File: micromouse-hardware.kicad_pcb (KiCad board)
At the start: 2 copper layers, 51 parts, among them Q1 MBT3904DW1, Q2 MBT3904DW1, Q3 MBT3904DW1, Q4 TEFT4300, Q5 TEFT4300, Q6 TEFT4300, Q7 TEFT4300, Q8 TEFT4300, SW1 SLW-116641-5A-S-D, SW2 SW_DIP_x02, U1 DRV8833PWPR, U2 74HC4051, U3 74HC238D, U4 MT3608

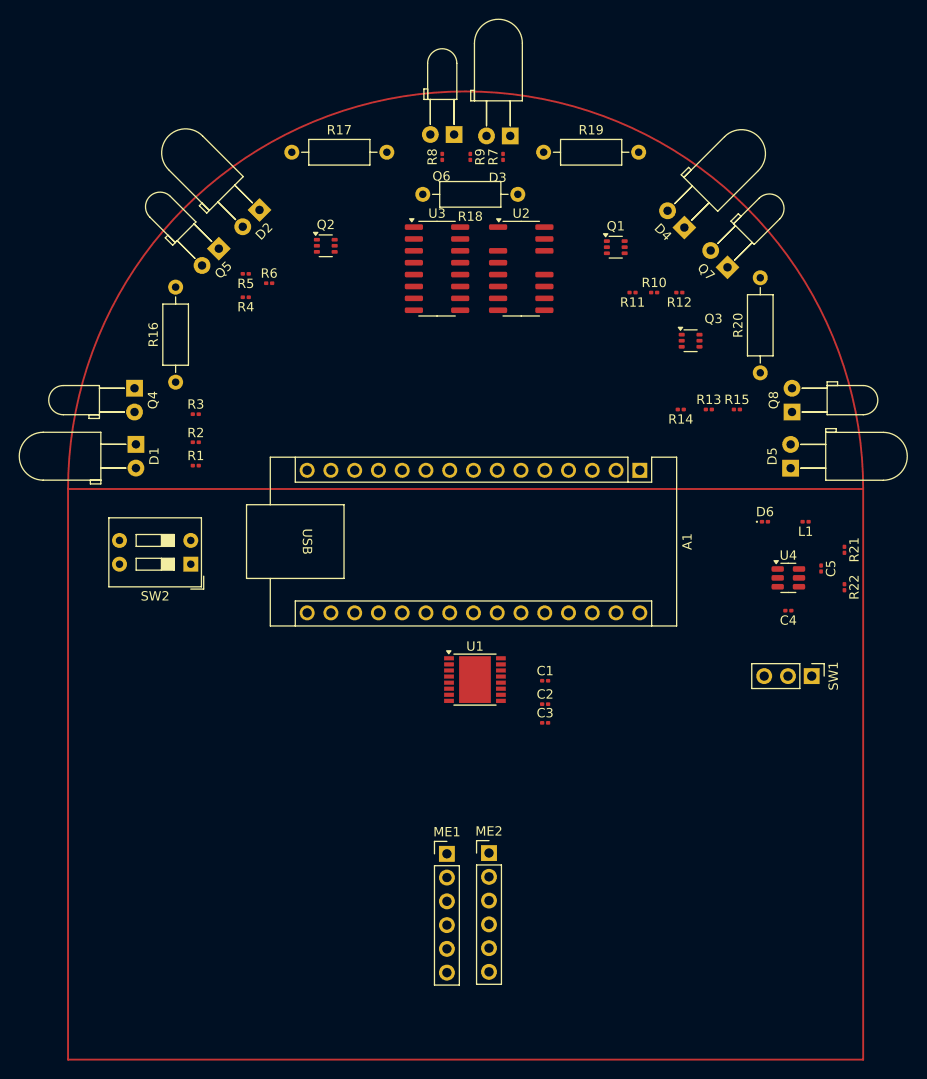
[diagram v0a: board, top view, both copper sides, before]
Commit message: second commit
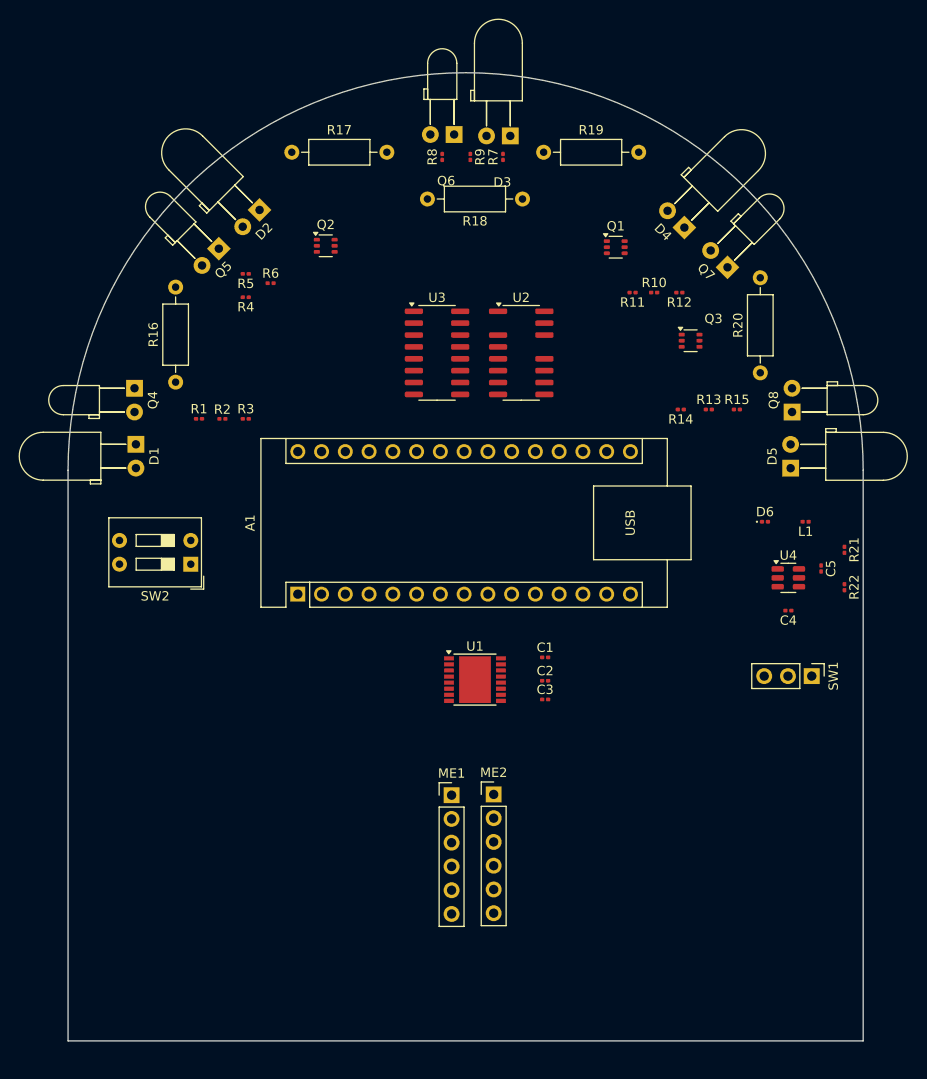
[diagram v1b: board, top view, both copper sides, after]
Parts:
- moved A1 38.9 mm to (132.1, 100.2), turned to 90 degrees
- moved U2 9.00 mm to (155.9, 74.4)
- moved U3 9.00 mm to (146.9, 74.4)
- moved ME1 6.29 mm to (148.5, 121.7)
- moved ME2 6.29 mm to (153.0, 121.7)
- moved R3 5.37 mm to (126.5, 81.5)
- moved R1 5.01 mm to (121.5, 81.5)
- moved R2 3.79 mm to (124.0, 81.5)
- moved C1 2.50 mm to (158.5, 107.0)
- moved C2 2.50 mm to (158.5, 109.5)
- moved C3 2.50 mm to (158.5, 111.5)
- moved R18 0.71 mm to (156.1, 58.0)
- moved R6 0.16 mm to (129.2, 67.0)
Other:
- board outline added: 85 x 103.5 mm
